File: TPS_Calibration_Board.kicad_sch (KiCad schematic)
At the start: 18 parts, among them J1 VEHICLE SIDE, J2 TPS SIDE, J3 PROG, P1 HID, U2 STM32G431K6Tx, U4 FT230XQ

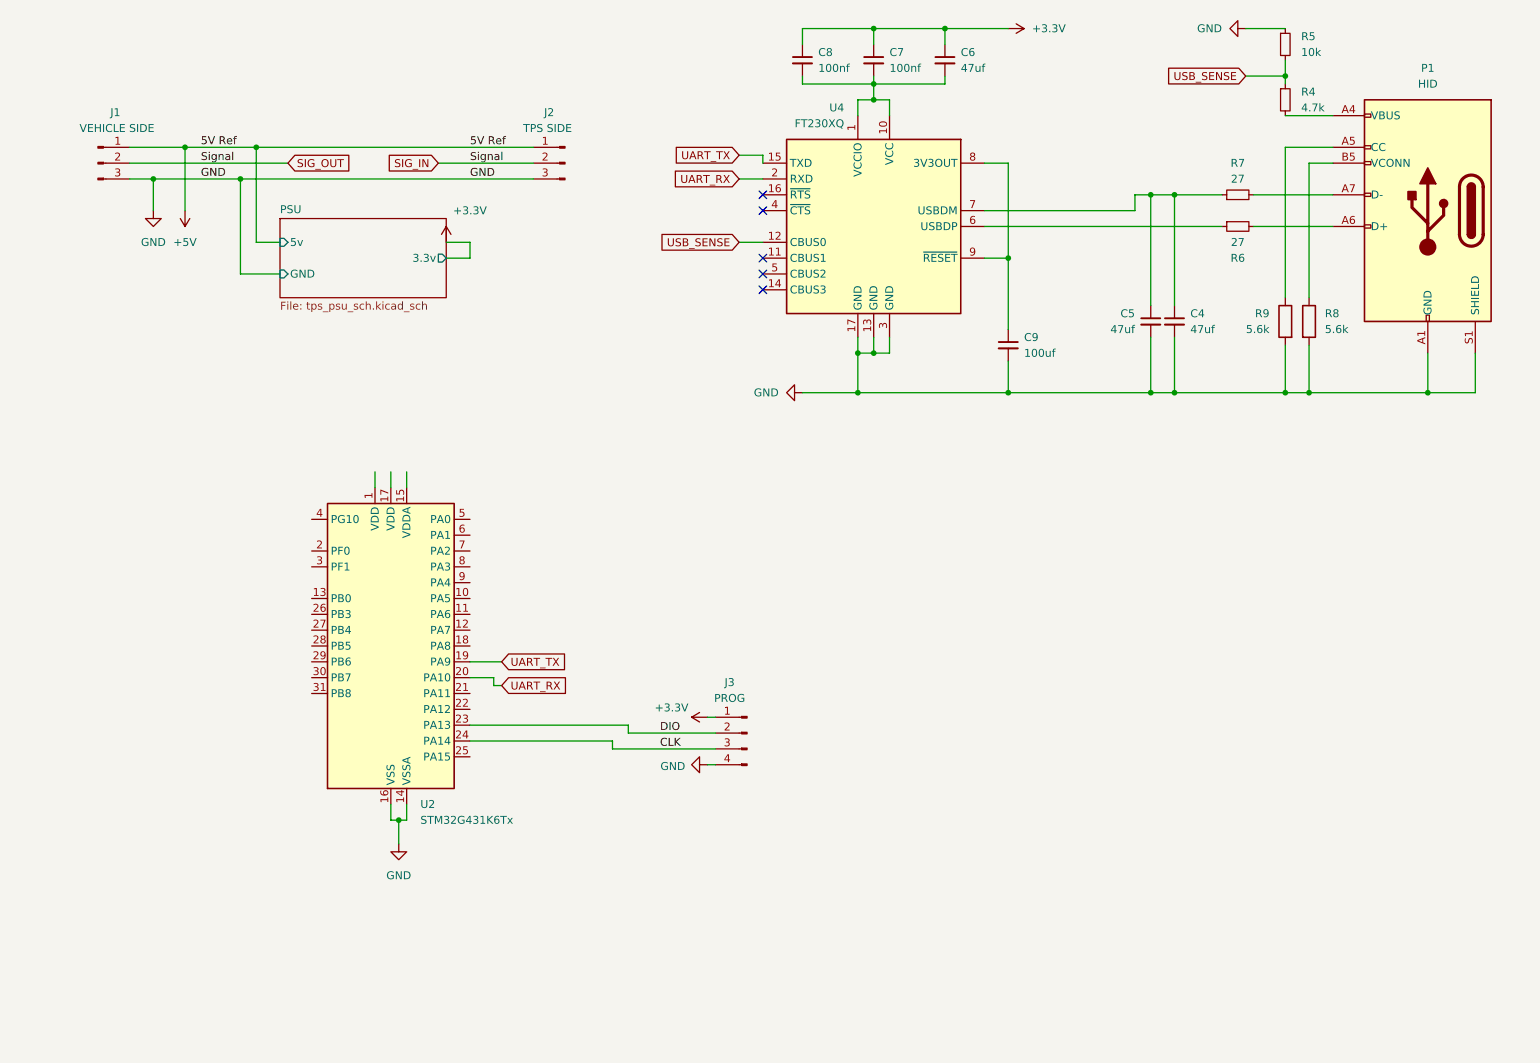
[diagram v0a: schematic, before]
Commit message: Finished board R00.
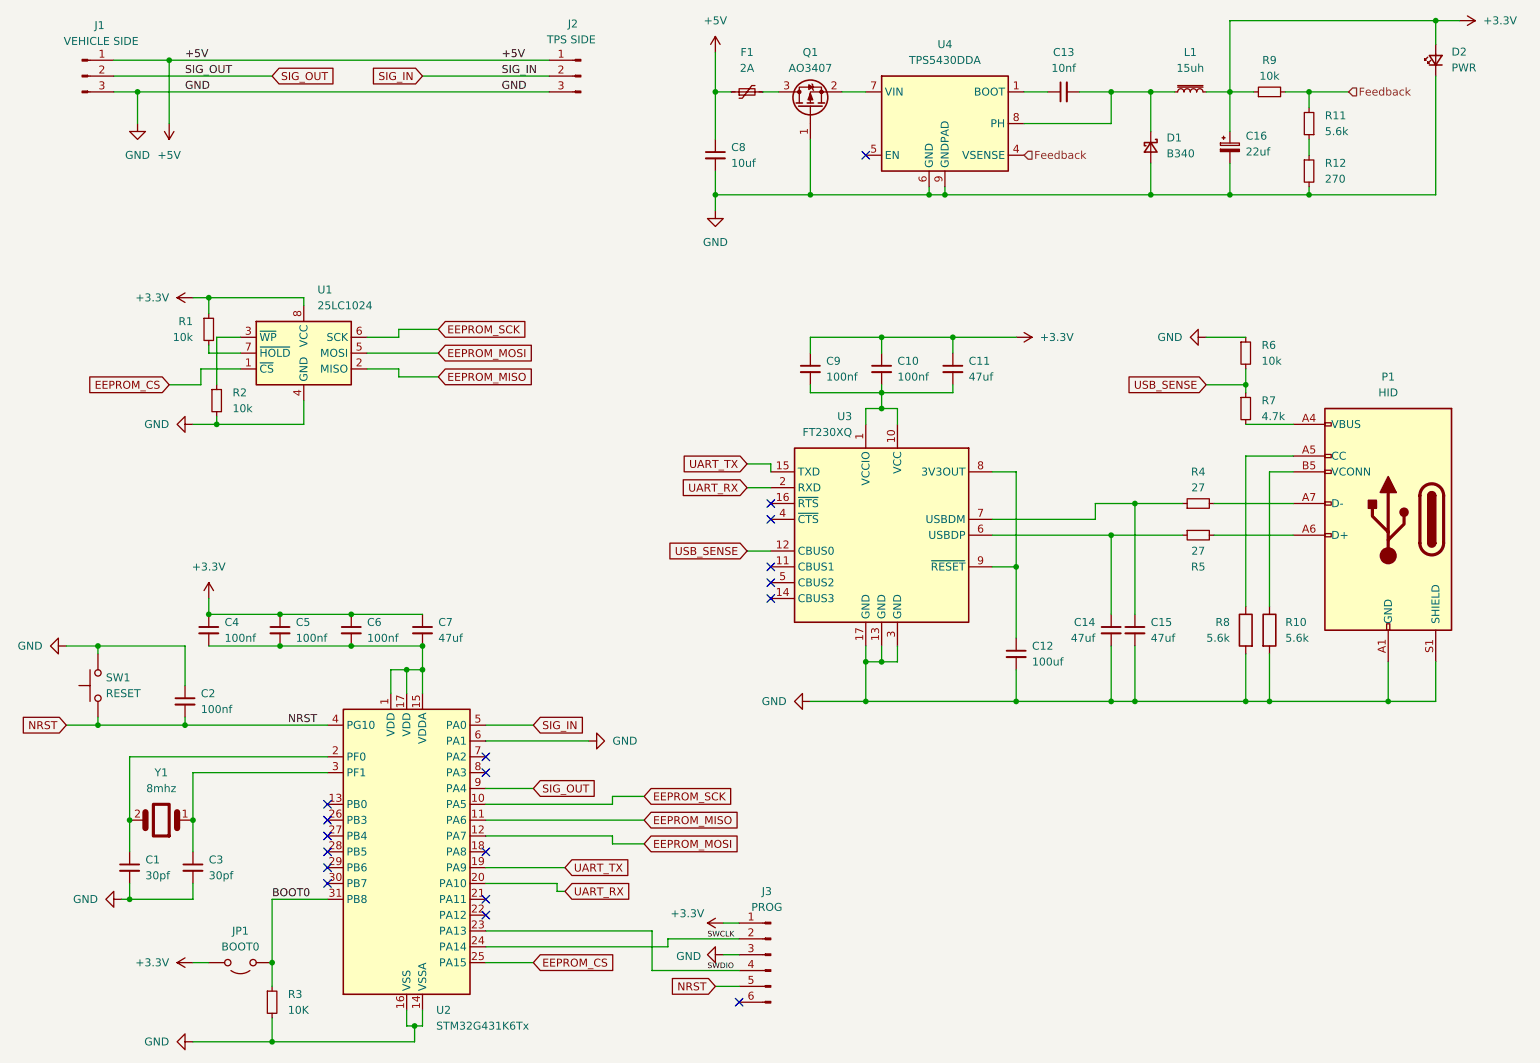
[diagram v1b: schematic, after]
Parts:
- removed J3: PROG, symbol Connector:Conn_01x04_Pin
- added C1, C3: 30pf, Capacitor_SMD:C_0805_2012Metric_Pad1.18x1.45mm_HandSolder, symbol Device:C_Small
- added C13: 10nf, Capacitor_SMD:C_0805_2012Metric_Pad1.18x1.45mm_HandSolder, symbol Device:C_Small
- added C16: 22uf, Capacitor_SMD:C_0805_2012Metric_Pad1.18x1.45mm_HandSolder, symbol Device:C_Polarized_Small
- added C2, C4, C5, C6: 100nf, Capacitor_SMD:C_0805_2012Metric_Pad1.18x1.45mm_HandSolder, symbol Device:C_Small
- added C7: 47uf, Capacitor_SMD:C_0805_2012Metric_Pad1.18x1.45mm_HandSolder, symbol Device:C_Small
- added C8: 10uf, Capacitor_SMD:C_0805_2012Metric_Pad1.18x1.45mm_HandSolder, symbol Device:C_Small
- added D1: B340, Diode_SMD:D_SMC_Handsoldering, symbol Device:D_Schottky_Small
- added D2: PWR, LED_SMD:LED_1206_3216Metric_Pad1.42x1.75mm_HandSolder, symbol Device:LED_Small
- added F1: 2A, Fuse:Fuse_0805_2012Metric_Pad1.15x1.40mm_HandSolder, symbol Device:Polyfuse_Small
- added J3: PROG, Connector_PinHeader_2.54mm:PinHeader_1x06_P2.54mm_Vertical, symbol Connector:Conn_01x06_Pin
- added JP1: BOOT0, Connector_PinHeader_2.54mm:PinHeader_1x03_P2.54mm_Vertical, symbol Jumper:Jumper_2_Open
- added L1: 15uh, Inductor_SMD:L_1210_3225Metric_Pad1.42x2.65mm_HandSolder, symbol Device:L_Iron_Small
- added Q1: AO3407, Package_TO_SOT_SMD:SOT-23, symbol Transistor_FET:AO3401A
- added R1, R2, R9: 10k, Resistor_SMD:R_1206_3216Metric_Pad1.30x1.75mm_HandSolder, symbol Device:R_Small
- added R11: 5.6k, Resistor_SMD:R_1206_3216Metric_Pad1.30x1.75mm_HandSolder, symbol Device:R_Small
- added R12: 270, Resistor_SMD:R_1206_3216Metric_Pad1.30x1.75mm_HandSolder, symbol Device:R_Small
- added R3: 10K, Resistor_SMD:R_1206_3216Metric_Pad1.30x1.75mm_HandSolder, symbol Device:R_Small
- added SW1: RESET, Button_Switch_SMD:SW_SPST_B3S-1000, symbol Switch:SW_Push
- added U1: 25LC1024, Package_DIP:DIP-8_W7.62mm_Socket, symbol Memory_EEPROM:25LCxxx
- added U4: TPS5430DDA, Package_SO:TI_SO-PowerPAD-8_ThermalVias, symbol Regulator_Switching:TPS5430DDA
- added Y1: 8mhz, Crystal:Crystal_HC49-4H_Vertical, symbol PCM_SL_Devices:Crystal_8MHz
- C10: renamed from C7; footprint (none) -> Capacitor_SMD:C_0805_2012Metric_Pad1.18x1.45mm_HandSolder
- C11: renamed from C6; footprint (none) -> Capacitor_SMD:C_0805_2012Metric_Pad1.18x1.45mm_HandSolder
- C12: renamed from C9; footprint (none) -> Capacitor_SMD:C_0805_2012Metric_Pad1.18x1.45mm_HandSolder
- C14: renamed from C5; footprint (none) -> Capacitor_SMD:C_0805_2012Metric_Pad1.18x1.45mm_HandSolder
- C15: renamed from C4; footprint (none) -> Capacitor_SMD:C_0805_2012Metric_Pad1.18x1.45mm_HandSolder
- C9: renamed from C8; footprint (none) -> Capacitor_SMD:C_0805_2012Metric_Pad1.18x1.45mm_HandSolder
- J1, J2: footprint (none) -> Connector_PinHeader_2.54mm:PinHeader_1x03_P2.54mm_Vertical
- P1: footprint (none) -> Connector_USB:USB_C_Receptacle_Molex_105450-0101
- R10: renamed from R8; footprint (none) -> Resistor_SMD:R_1206_3216Metric_Pad1.30x1.75mm_HandSolder
- R4: renamed from R7; footprint (none) -> Resistor_SMD:R_1206_3216Metric_Pad1.30x1.75mm_HandSolder
- R5: renamed from R6; footprint (none) -> Resistor_SMD:R_1206_3216Metric_Pad1.30x1.75mm_HandSolder
- R6: renamed from R5; footprint (none) -> Resistor_SMD:R_1206_3216Metric_Pad1.30x1.75mm_HandSolder
- R7: renamed from R4; footprint (none) -> Resistor_SMD:R_1206_3216Metric_Pad1.30x1.75mm_HandSolder
- R8: renamed from R9; footprint (none) -> Resistor_SMD:R_1206_3216Metric_Pad1.30x1.75mm_HandSolder
- renumbered U4 to U3
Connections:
- net +3.3V: now also C16.1, C4.1, C5.1, C6.1, C7.1, D2.2 (A), J3.1 (Pin_1), JP1.2 (B), L1.2, R1.1, R9.1, U1.8 (VCC)
- net +5V: now also C8.1, F1.1
- net GND: now also U2.6 (PA1), C1.2, C16.2, C2.1, C3.2, C8.2, D1.2 (A), D2.1 (K), J3.3 (Pin_3), Q1.1 (G), R12.2, R2.2, R3.2, SW1.2, U1.4 (GND), U4.6 (GND), U4.9 (GNDPAD)
- net SIG_IN: now also U2.5 (PA0); no longer J1.2 (Pin_2)
- net at R5.1, U3.6 (USBDP): now also C14.1
- net at C15.1, R4.1, U3.7 (USBDM): no longer C14.1
- net at U2.1 (VDD): now also U2.15 (VDDA), U2.17 (VDD), C4.2, C5.2, C6.2, C7.2
- net EEPROM_SCK: now reaches U2.10 (PA5)
- net EEPROM_SCK: now also U1.6 (SCK)
- net EEPROM_MISO: now reaches U2.11 (PA6)
- net EEPROM_MISO: now also U1.2 (MISO)
- net EEPROM_MOSI: now reaches U2.12 (PA7)
- net EEPROM_MOSI: now also U1.5 (MOSI)
- net at U2.2 (PF0): now also C1.1, Y1.2
- net EEPROM_CS: now reaches U2.25 (PA15)
- net EEPROM_CS: now also U1.1 (~{CS})
- net at U2.3 (PF1): now also C3.1, Y1.1
- net BOOT0: now reaches U2.31 (PB8)
- net BOOT0: now also JP1.1 (A), R3.1
- net NRST: now reaches U2.4 (PG10)
- net NRST: now also C2.2, J3.5 (Pin_5), SW1.1
- net SIG_OUT: now reaches U2.9 (PA4)
- net SIG_OUT: now also J1.2 (Pin_2)
- net CLK renamed SWCLK
- net SWCLK: now also J3.2 (Pin_2)
- net DIO renamed SWDIO
- net SWDIO: now also J3.4 (Pin_4)
- new net: R11.1, R12.1
- new net: Q1.2 (S), U4.7 (VIN)
- new net: F1.2, Q1.3 (D)
- new net: R2.1, U1.3 (~{WP})
- new net: R1.2, U1.7 (~{HOLD})
- new net: C13.1, U4.1 (BOOT)
- new net: C13.2, D1.1 (K), L1.1, U4.8 (PH)
- new net Feedback: R11.2, R9.2, U4.4 (VSENSE)
- no-connect marks 5 -> 18
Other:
- removed sheet PSU
- company: (none) -> R.U.I
- title: (none) -> Cable TPS Calibration System
- moved on the sheet: C10, C11, C12, C14, C15, C9, J1, J2, P1, R10, R4, R5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
